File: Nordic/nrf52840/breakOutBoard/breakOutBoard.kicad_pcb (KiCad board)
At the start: 4 copper layers, 30 x 26.8 mm, 24 parts, among them J1 Conn_ARM_JTAG_SWD_10, U1 NRF52840-QFAA-R7, Y1 Crystal, Y2 ECS-327MVATX-3-CN-TR3

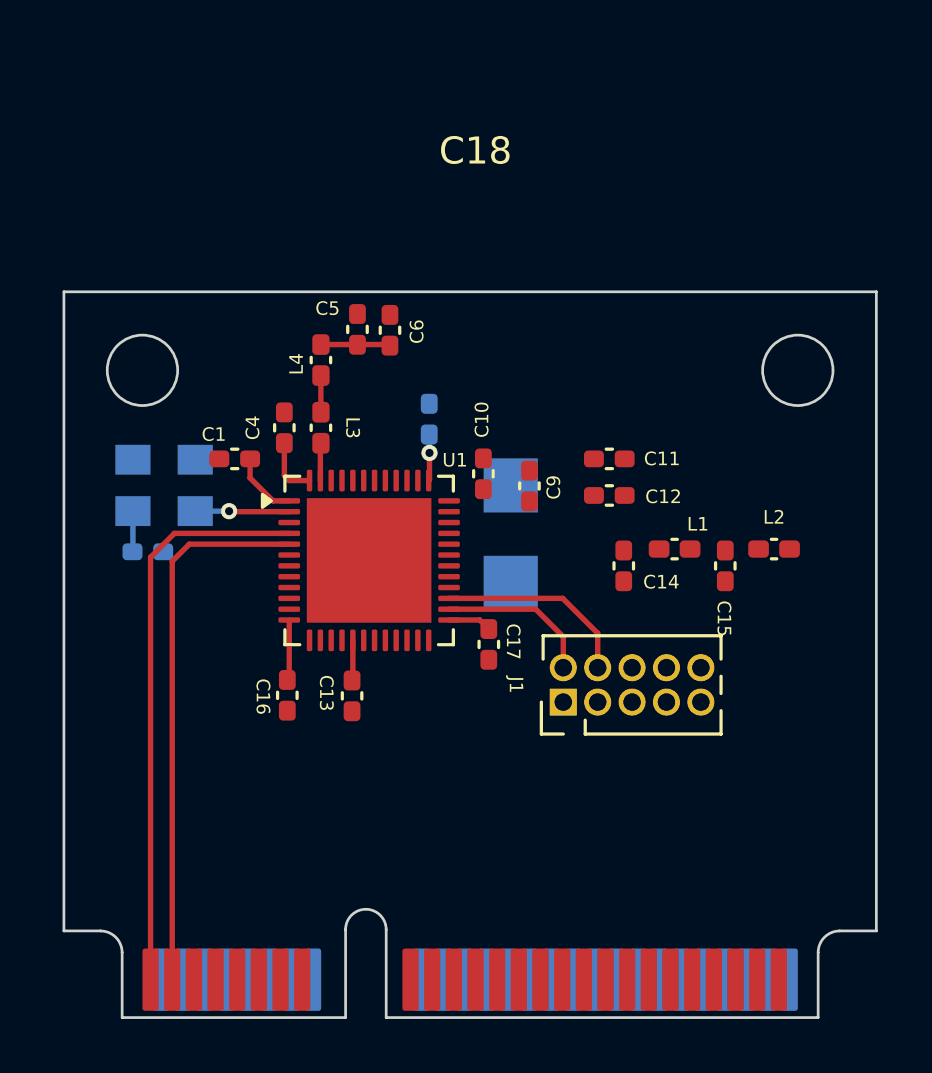
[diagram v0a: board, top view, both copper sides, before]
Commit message: projects
Update projects
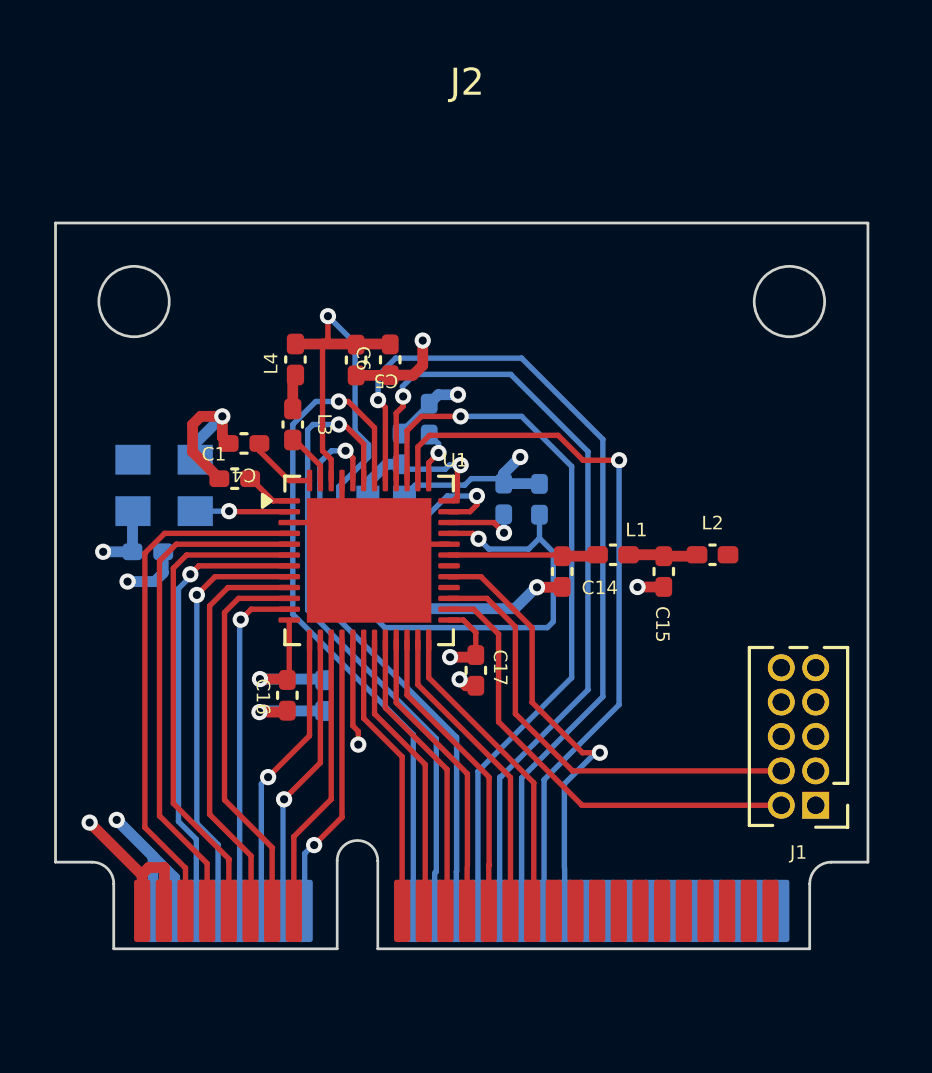
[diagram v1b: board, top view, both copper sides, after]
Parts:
- C10, C11, C12, C13, C9: moved to B.Cu
- Y1: value Crystal -> ECS-320-8-37B-CKY-TR; footprint Crystal:Crystal_SMD_Qantek_QC5CB-2Pin_5x3.2mm -> User_Footprint:XTAL_ECS-160-9-37-CKM-TR
- moved J1 10.1 mm to (170.8, 90.7), turned to 180 degrees
- moved C9 5.84 mm to (155.1, 81.6), turned to 0 degrees
- moved Y1 4.69 mm to (154.9, 79.8), turned to 0 degrees
- moved C12 3.90 mm to (159.3, 79.3), turned to 90 degrees
- moved C10 3.18 mm to (155.5, 77.5), turned to -90 degrees
- moved C11 2.98 mm to (160.6, 79.4), turned to 90 degrees
- moved J2 2.56 mm to (157.9, 81.0)
- moved C14 2.28 mm to (161.4, 82.0)
- moved C15 2.28 mm to (165.2, 82.0)
- moved L1 2.28 mm to (163.3, 81.4)
- moved L2 2.28 mm to (167.0, 81.4)
- moved C4 1.60 mm to (149.7, 77.3), turned to 180 degrees
- moved C5 1.13 mm to (153.8, 74.2), turned to -90 degrees
- moved C6 1.09 mm to (155.1, 74.2), turned to -90 degrees
- moved C17 1.07 mm to (158.3, 85.7)
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- renumbered C18 to J2
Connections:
- C10 pad 1: Net-(U1-XC2) -> GND
- C10 pad 2: GND -> /XC1
- C9 pad 1: Net-(U1-XC1) -> GND
- C9 pad 2: GND -> /XC2
- J2 pad 1: unconnected-(C18-Pad1) -> VDD
- J2 pad 10: unconnected-(C18-Pad10) -> /P0.12
- J2 pad 11: unconnected-(C18-Pad11) -> /P1.09
- J2 pad 12: unconnected-(C18-Pad12) -> /P0.13
- J2 pad 13: unconnected-(C18-Pad13) -> /P0.11
- J2 pad 14: unconnected-(C18-Pad14) -> /P0.14
- J2 pad 15: unconnected-(C18-Pad15) -> /P0.17
- J2 pad 16: unconnected-(C18-Pad16) -> /P0.18
- J2 pad 17: unconnected-(C18-Pad17) -> /P0.19
- J2 pad 18: unconnected-(C18-Pad18) -> /P0.29
- J2 pad 19: unconnected-(C18-Pad19) -> /P0.20
- J2 pad 2: unconnected-(C18-Pad2) -> GND
- J2 pad 20: unconnected-(C18-Pad20) -> /P0.30
- J2 pad 21: unconnected-(C18-Pad21) -> /P0.21
- J2 pad 22: unconnected-(C18-Pad22) -> /P0.31
- J2 pad 23: unconnected-(C18-Pad23) -> /P0.22
- J2 pad 24: unconnected-(C18-Pad24) -> /P0.03
- J2 pad 25: unconnected-(C18-Pad25) -> /P0.23
- J2 pad 26: unconnected-(C18-Pad26) -> /P0.02
- J2 pad 27: unconnected-(C18-Pad27) -> /P0.24
- J2 pad 28: unconnected-(C18-Pad28) -> /P0.28
- J2 pad 29: unconnected-(C18-Pad29) -> /P1.00
- J2 pad 3: unconnected-(C18-Pad3) -> VDD
- J2 pad 30: unconnected-(C18-Pad30) -> /P1.15
- J2 pad 31: unconnected-(C18-Pad31) -> /P0.09
- J2 pad 32: unconnected-(C18-Pad32) -> /P0.09
- J2 pad 4: unconnected-(C18-Pad4) -> GND
- J2 pad 5: unconnected-(C18-Pad5) -> /P0.04
- J2 pad 6: unconnected-(C18-Pad6) -> /P0.08
- J2 pad 7: unconnected-(C18-Pad7) -> /P0.05
- J2 pad 8: unconnected-(C18-Pad8) -> /P1.08
- J2 pad 9: unconnected-(C18-Pad9) -> /P0.07
- U1 pad 35: Net-(U1-XC1) -> /XC2
- U1 pad 36: Net-(U1-XC2) -> /XC1
- Y1 pad 1: Net-(U1-XC2) -> /XC1
- Y1 pad 2: Net-(U1-XC1) -> GND
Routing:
- net GND: track 0.00 -> 50.1 mm, vias 0 -> 10
- net Net-(U1-DEC4): track 2.57 -> 37.3 mm, vias 0 -> 2
- net /P0.28: track 0.00 -> 32.4 mm, vias 0 -> 1
- net /P0.02: track 0.00 -> 30.1 mm, vias 0 -> 1
- net /P1.15: track 0.00 -> 27.0 mm, vias 0 -> 1
- net /P0.03: track 0.00 -> 26.7 mm, vias 0 -> 1
- net /P0.29: track 0.00 -> 25.5 mm, vias 0 -> 1
- net /P0.30: track 0.00 -> 23.6 mm, vias 0 -> 1
- net /P0.31: track 0.00 -> 21.0 mm, vias 0 -> 1
- net /P0.07: track 0.00 -> 18.0 mm
- net /P0.08: track 0.00 -> 16.8 mm, vias 0 -> 1
- net /P0.09: track 0.00 -> 16.3 mm, vias 0 -> 1
- net /P1.08: track 0.00 -> 15.7 mm, vias 0 -> 1
- net VDD: track 10.8 -> 26.0 mm, vias 1 -> 6
- net /P1.09: track 0.00 -> 15.1 mm
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- added copper zone on In1.Cu, net GND
- added copper zone on In2.Cu, net VDD
